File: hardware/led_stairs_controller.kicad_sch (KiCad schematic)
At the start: 87 parts, among them J1 Conn_01x05_Socket, J2 Conn_01x04_Pin, J3 Conn_01x05_Pin, Q1 QM6006D, Q10 QM6006D, Q11 QM6006D, Q12 QM6006D, Q13 QM6006D, Q14 QM6006D, Q15 QM6006D, Q16 QM6006D, Q17 BSS138, Q18 BSS138, Q19 BSS138, Q2 QM6006D, Q3 QM6006D, Q4 QM6006D, Q5 QM6006D, Q6 QM6006D, Q7 QM6006D, Q8 QM6006D, Q9 QM6006D, U1 PCA9635, U2 ESP32-DEVKITC-32UE, U3 PC817, U4 MCP23008-xSO, U5 PC817, U6 PC817, U7 PC817, U8 R-78E5.0-1.0

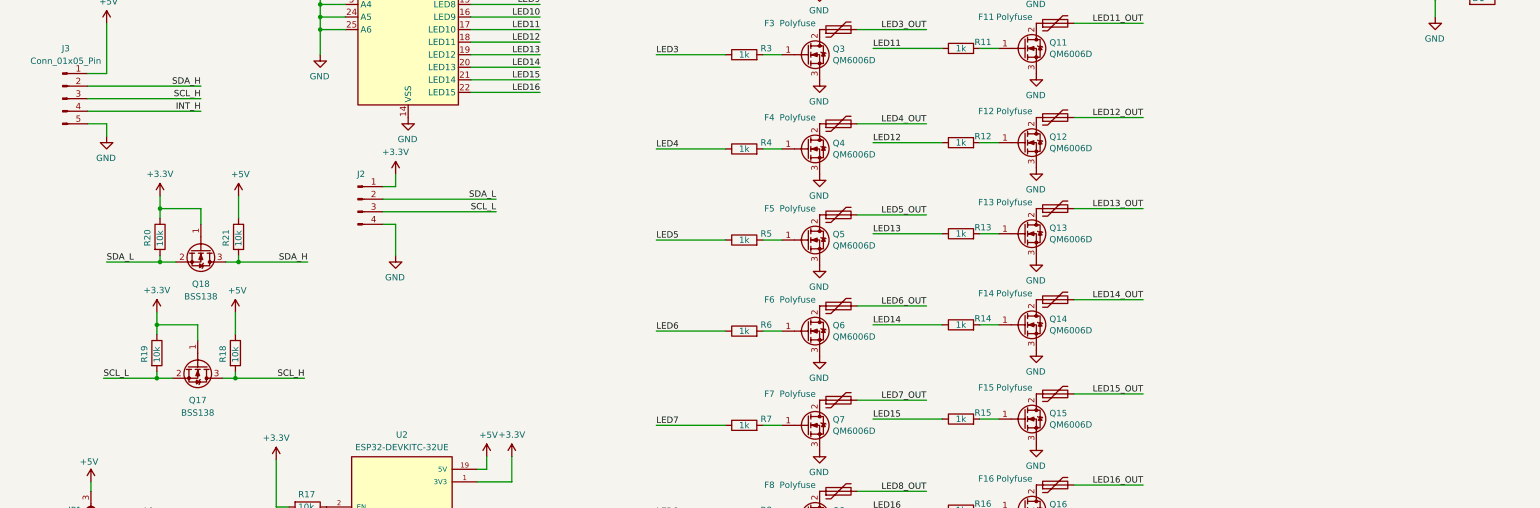
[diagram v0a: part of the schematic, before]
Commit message: update
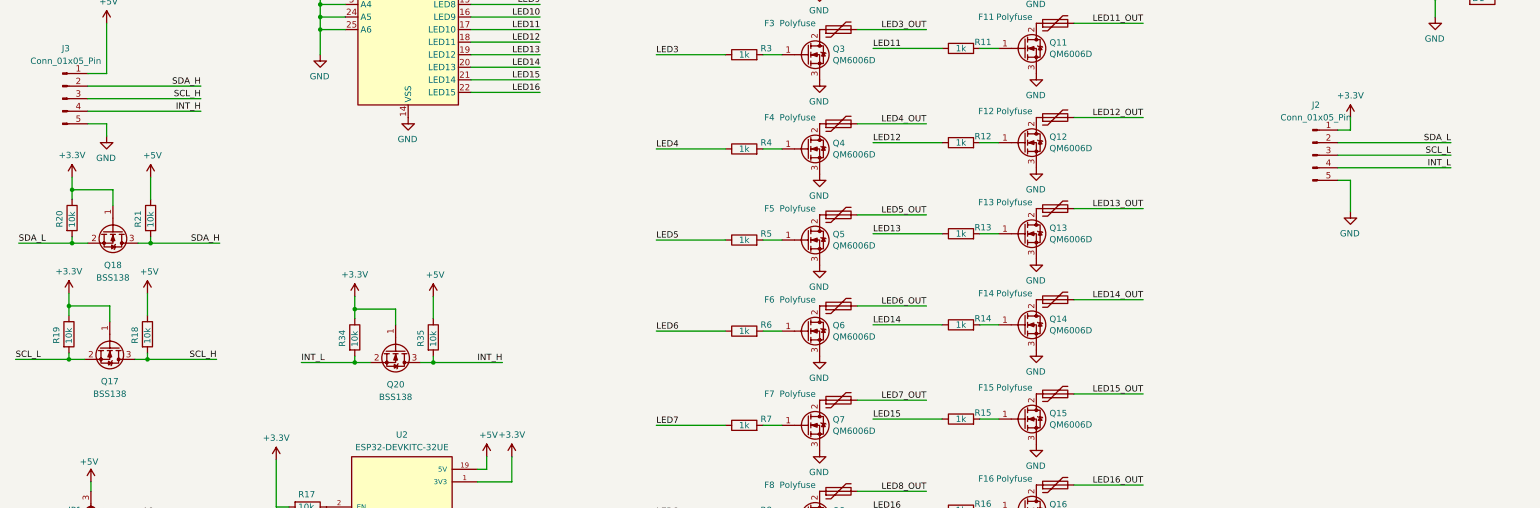
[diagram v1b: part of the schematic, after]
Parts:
- added Q20: BSS138, Package_TO_SOT_SMD:SOT-23, symbol Transistor_FET:BSS138
- added R34, R35: R0603_10k_1%_100mW_100PPM_AC, Resistor_SMD:R_0603_1608Metric, symbol Resistors_SMD_0603:R0603_10k_1%_100mW_100PPM_AC
- J2: value Conn_01x04_Pin -> Conn_01x05_Pin; footprint Connector_PinHeader_2.54mm:PinHeader_1x04_P2.54mm_Vertical -> Connector_PinHeader_2.54mm:PinHeader_1x05_P2.54mm_Vertical; symbol Connector:Conn_01x04_Pin -> Connector:Conn_01x05_Pin
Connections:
- net +3.3V: now also Q20.1 (G), R34.1
- net +5V: now also R35.1
- net GND: now also J2.5 (Pin_5); no longer J2.4 (Pin_4)
- net INT_H: now also Q20.3 (D), R35.2
- new net INT_L: J2.4 (Pin_4), Q20.2 (S), R34.2
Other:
- moved on the sheet: Q17, Q18, R18, R19, R20, R21
